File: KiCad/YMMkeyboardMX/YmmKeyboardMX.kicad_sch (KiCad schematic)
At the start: 66 parts, among them J4 OLED, J5 RGB, J6 汎用5ピン, SW00 SW_Push, SW01 SW_Push, SW02 SW_Push, SW03 SW_Push, SW04 SW_Push, SW05 SW_Push, SW10 SW_Push, SW11 SW_Push, SW12 SW_Push, SW13 SW_Push, SW14 SW_Push, SW15 SW_Push, SW20 SW_Push, SW22 SW_Push, SW23 SW_Push, SW24 SW_Push, SW25 SW_Push, SW30 SW_Push, SW31 SW_Push, SW32 SW_Push, SW33 SW_Push, SW34 SW_Push, SW35 SW_Push, SW40 SW_Push, SW41 SW_Push, SW42 SW_Push, SW43 SW_Push, SW44 SW_Push, SW45 SW_Push, SW56 RotaryEncoder_Switch, U1 RP2040-Zero

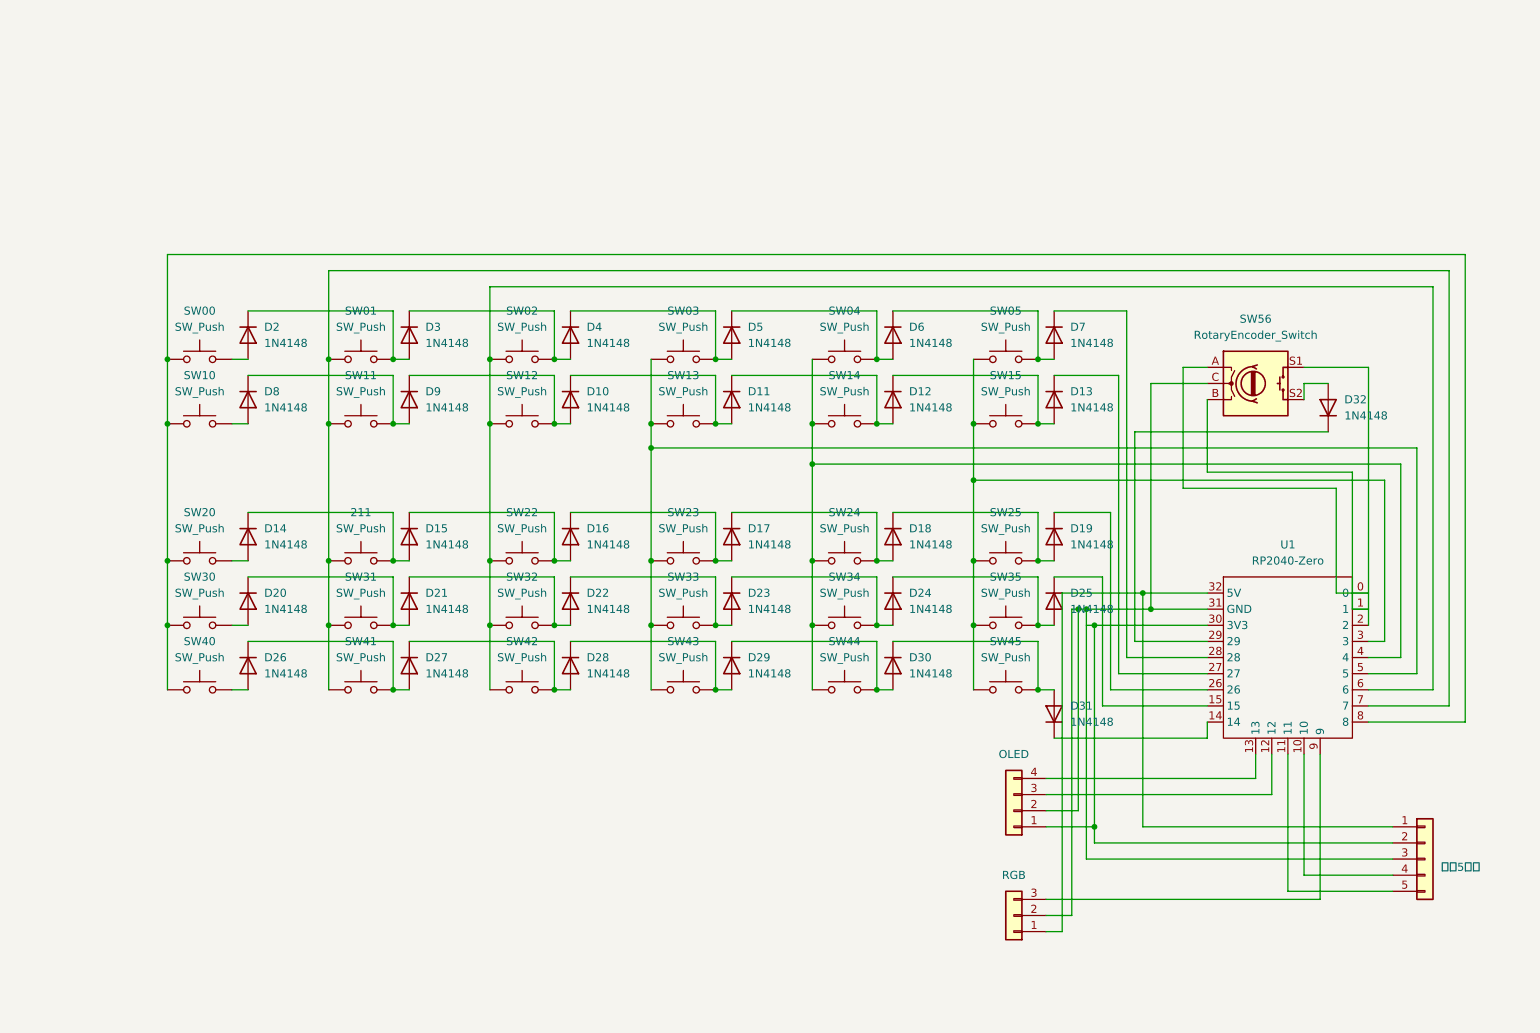
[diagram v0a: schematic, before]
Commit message: キーボード完成 LED追加するべき？
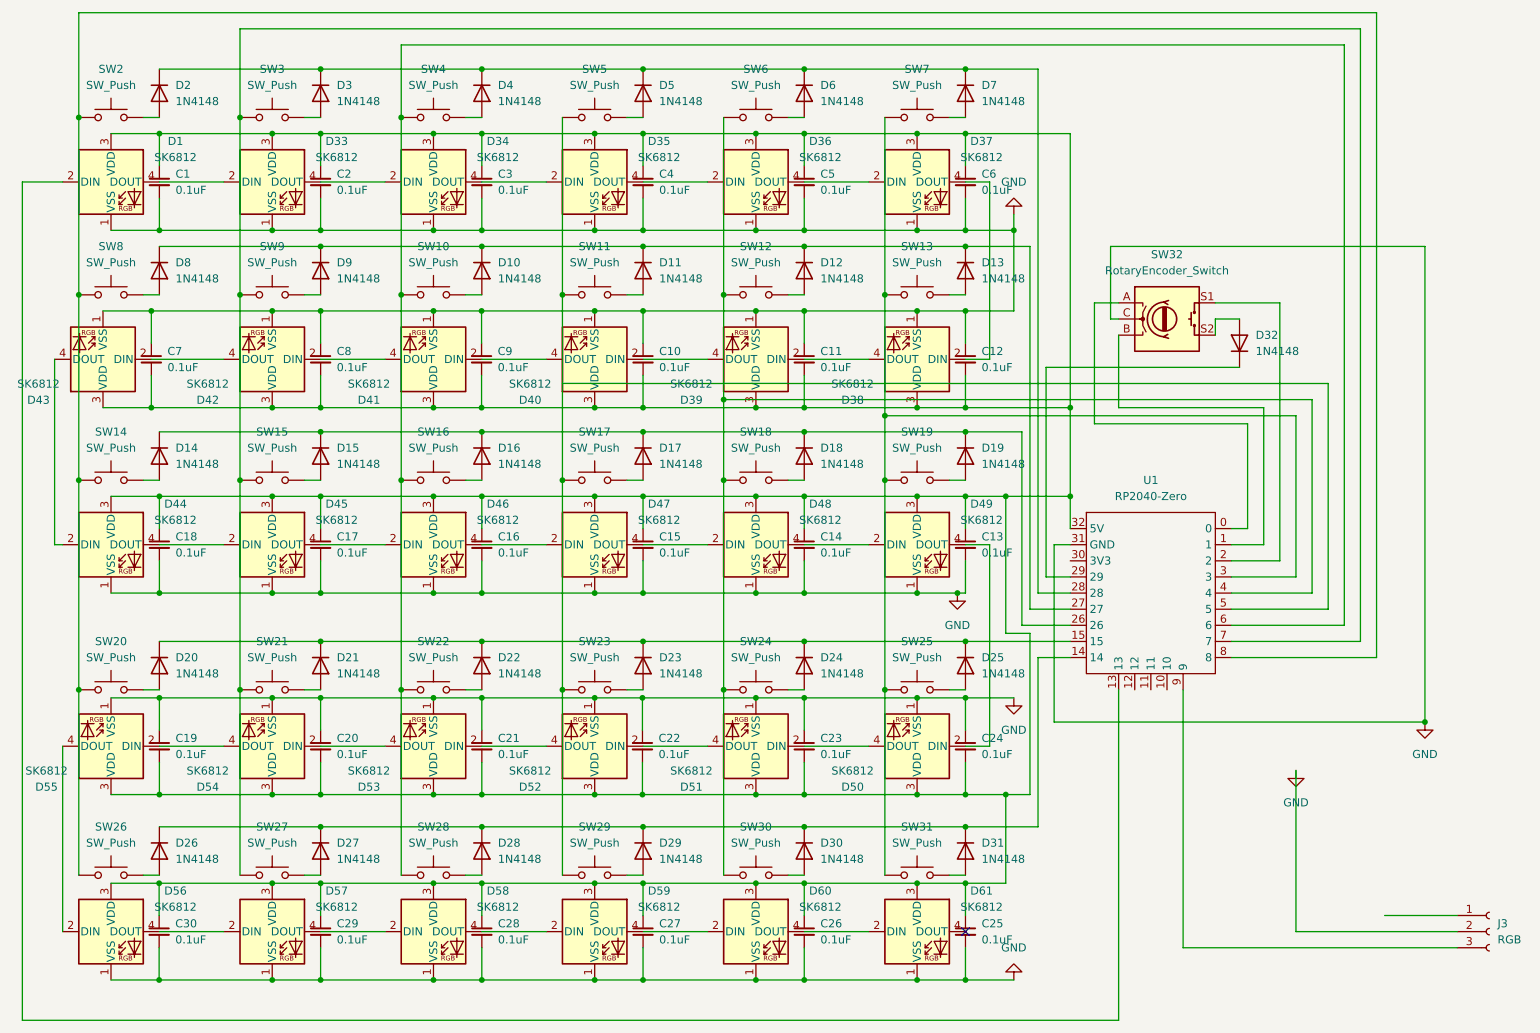
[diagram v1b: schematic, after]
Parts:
- removed J4: OLED, Connector_PinSocket_2.54mm:PinSocket_1x04_P2.54mm_Vertical, symbol Connector_Generic:Conn_01x04
- removed J5: RGB, Connector_PinSocket_2.54mm:PinSocket_1x03_P2.54mm_Vertical, symbol Connector_Generic:Conn_01x03
- removed J6: 汎用5ピン, Connector_PinSocket_2.54mm:PinSocket_1x05_P2.54mm_Vertical, symbol Connector_Generic:Conn_01x05
- added C1, C10, C11, C12, C13, C14, C15, C16, C17, C18, C19, C2, C20, C21, C22, C23, C24, C25, C26, C27, C28, C29, C3, C30, C4, C5, C6, C7, C8, C9: 0.1uF, Capacitor_SMD:C_0603_1608Metric_Pad1.08x0.95mm_HandSolder, symbol Device:C_Small
- added D1, D33, D34, D35, D36, D37, D38, D39, D40, D41, D42, D43, D44, D45, D46, D47, D48, D49, D50, D51, D52, D53, D54, D55, D56, D57, D58, D59, D60, D61: SK6812, LED_SMD:LED_SK6812_PLCC4_5.0x5.0mm_P3.2mm, symbol LED:SK6812
- added J3: RGB, Connector_PinSocket_2.54mm:PinSocket_1x03_P2.54mm_Vertical, symbol Connector:Conn_01x03_Socket
- renumbered SW12 to SW10, SW13 to SW11, SW14 to SW12, SW15 to SW13, SW20 to SW14, 211 to SW15, SW22 to SW16, SW23 to SW17, SW24 to SW18, SW25 to SW19, SW00 to SW2, SW30 to SW20, SW31 to SW21, SW32 to SW22, SW33 to SW23, SW34 to SW24, SW35 to SW25, SW40 to SW26, SW41 to SW27, SW42 to SW28, SW43 to SW29, SW01 to SW3, SW44 to SW30, SW45 to SW31, SW56 to SW32, SW02 to SW4, SW03 to SW5, SW04 to SW6, SW05 to SW7, SW10 to SW8, SW11 to SW9
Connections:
- net at D19.2 (A), SW19.2: no longer D18.1 (K)
- net at D27.2 (A), SW27.2: no longer D26.1 (K)
- net at D25.2 (A), SW25.2: no longer D24.1 (K)
- net GND: now reaches SW32.C, U1.31 (GND)
- net GND: now also C1.2, C10.1, C11.1, C12.1, C13.2, C14.2, C15.2, C16.2, C17.2, C18.2, C19.1, C2.2, C20.1, C21.1, C22.1, C23.1, C24.1, C25.2, C26.2, C27.2, C28.2, C29.2, C3.2, C30.2, C4.2, C5.2, C6.2, C7.1, C8.1, C9.1, D1.1 (VSS), D33.1 (VSS), D34.1 (VSS), D35.1 (VSS), D36.1 (VSS), D37.1 (VSS), D38.1 (VSS), D39.1 (VSS), D40.1 (VSS), D41.1 (VSS), D42.1 (VSS), D43.1 (VSS), D44.1 (VSS), D45.1 (VSS), D46.1 (VSS), D47.1 (VSS), D48.1 (VSS), D49.1 (VSS), D50.1 (VSS), D51.1 (VSS), D52.1 (VSS), D53.1 (VSS), D54.1 (VSS), D55.1 (VSS), D56.1 (VSS), D57.1 (VSS), D58.1 (VSS), D59.1 (VSS), D60.1 (VSS), D61.1 (VSS), J3.2 (Pin_2)
- net at D7.2 (A), SW7.2: no longer D6.1 (K)
- net at D30.2 (A), SW30.2: no longer D29.1 (K)
- net at D29.2 (A), SW29.2: no longer D28.1 (K)
- net at D31.2 (A), SW31.2: no longer D30.1 (K)
- net at D11.2 (A), SW11.2: no longer D10.1 (K)
- net at D7.1 (K), U1.28: now also D2.1 (K), D3.1 (K), D4.1 (K), D5.1 (K), D6.1 (K)
- net at D6.2 (A), SW6.2: no longer D5.1 (K)
- net at D5.2 (A), SW5.2: no longer D4.1 (K)
- net at D10.2 (A), SW10.2: no longer D9.1 (K)
- net at D9.2 (A), SW9.2: no longer D8.1 (K)
- net at D31.1 (K), U1.14: now also D26.1 (K), D27.1 (K), D28.1 (K), D29.1 (K), D30.1 (K)
- net at D4.2 (A), SW4.2: no longer D3.1 (K)
- net at D23.2 (A), SW23.2: no longer D22.1 (K)
- net at D3.2 (A), SW3.2: no longer D2.1 (K)
- net at U1.13: now also D1.2 (DIN)
- net at D25.1 (K), U1.15: now also D20.1 (K), D21.1 (K), D22.1 (K), D23.1 (K), D24.1 (K)
- net at D19.1 (K), U1.26: now also D14.1 (K), D15.1 (K), D16.1 (K), D17.1 (K), D18.1 (K)
- net at D13.1 (K), U1.27: now also D10.1 (K), D11.1 (K), D12.1 (K), D8.1 (K), D9.1 (K)
- net at U1.32 (5V): now also C1.1, C10.2, C11.2, C12.2, C13.1, C14.1, C15.1, C16.1, C17.1, C18.1, C19.2, C2.1, C20.2, C21.2, C22.2, C23.2, C24.2, C25.1, C26.1, C27.1, C28.1, C29.1, C3.1, C30.1, C4.1, C5.1, C6.1, C7.2, C8.2, C9.2, D1.3 (VDD), D33.3 (VDD), D34.3 (VDD), D35.3 (VDD), D36.3 (VDD), D37.3 (VDD), D38.3 (VDD), D39.3 (VDD), D40.3 (VDD), D41.3 (VDD), D42.3 (VDD), D43.3 (VDD), D44.3 (VDD), D45.3 (VDD), D46.3 (VDD), D47.3 (VDD), D48.3 (VDD), D49.3 (VDD), D50.3 (VDD), D51.3 (VDD), D52.3 (VDD), D53.3 (VDD), D54.3 (VDD), D55.3 (VDD), D56.3 (VDD), D57.3 (VDD), D58.3 (VDD), D59.3 (VDD), D60.3 (VDD), D61.3 (VDD)
- net at U1.9: now also J3.3 (Pin_3)
- net at D13.2 (A), SW13.2: no longer D12.1 (K)
- net at D16.2 (A), SW16.2: no longer D15.1 (K)
- net at D21.2 (A), SW21.2: no longer D20.1 (K)
- net at D24.2 (A), SW24.2: no longer D23.1 (K)
- net at D18.2 (A), SW18.2: no longer D17.1 (K)
- net at D22.2 (A), SW22.2: no longer D21.1 (K)
- net at D15.2 (A), SW15.2: no longer D14.1 (K)
- net at D12.2 (A), SW12.2: no longer D11.1 (K)
- net at D17.2 (A), SW17.2: no longer D16.1 (K)
- net at D28.2 (A), SW28.2: no longer D27.1 (K)
- new net: D45.4 (DOUT), D46.2 (DIN)
- new net: D46.4 (DOUT), D47.2 (DIN)
- new net: D55.4 (DOUT), D56.2 (DIN)
- new net: D56.4 (DOUT), D57.2 (DIN)
- new net: D37.4 (DOUT), D38.2 (DIN)
- new net: D38.4 (DOUT), D39.2 (DIN)
- new net: D40.4 (DOUT), D41.2 (DIN)
- new net: D41.4 (DOUT), D42.2 (DIN)
- new net: D44.4 (DOUT), D45.2 (DIN)
- new net: D1.4 (DOUT), D33.2 (DIN)
- new net: D49.4 (DOUT), D50.2 (DIN)
- new net: D50.4 (DOUT), D51.2 (DIN)
- new net: D42.4 (DOUT), D43.2 (DIN)
- new net: D43.4 (DOUT), D44.2 (DIN)
- new net: D51.4 (DOUT), D52.2 (DIN)
- new net: D58.4 (DOUT), D59.2 (DIN)
- new net: D59.4 (DOUT), D60.2 (DIN)
- new net: D52.4 (DOUT), D53.2 (DIN)
- new net: D53.4 (DOUT), D54.2 (DIN)
- new net: D36.4 (DOUT), D37.2 (DIN)
- new net: D39.4 (DOUT), D40.2 (DIN)
- new net: D60.4 (DOUT), D61.2 (DIN)
- new net: D33.4 (DOUT), D34.2 (DIN)
- new net: D34.4 (DOUT), D35.2 (DIN)
- new net: D47.4 (DOUT), D48.2 (DIN)
- new net: D48.4 (DOUT), D49.2 (DIN)
- new net: D57.4 (DOUT), D58.2 (DIN)
- new net: D35.4 (DOUT), D36.2 (DIN)
- new net: D54.4 (DOUT), D55.2 (DIN)
- no-connect marks 0 -> 1
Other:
- moved on the sheet: D10, D11, D12, D13, D14, D15, D16, D17, D18, D19, D2, D20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
